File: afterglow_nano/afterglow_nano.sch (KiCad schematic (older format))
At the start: 64 parts, among them J1 J137_IN_C, J2 J133_IN_R, J3 Conn_Power, J4 J137_OUT_C, J5 J133_OUT_R, Q1 2N3904, Q10 FQP27P06, Q11 FQP27P06, Q12 FQP27P06, Q13 FQP27P06, Q14 FQP27P06, Q15 FQP27P06, Q16 FQP27P06, Q17 FQP30N06L, Q18 FQP30N06L, Q19 FQP30N06L, Q2 2N3904, Q20 FQP30N06L, Q21 FQP30N06L, Q22 FQP30N06L, Q23 FQP30N06L, Q24 FQP30N06L, Q3 2N3904, Q4 2N3904, Q5 2N3904, Q6 2N3904, Q7 2N3904, Q8 2N3904, Q9 FQP27P06, SW1 CFG, U1 74LS165, U2 74LS165, U3 5V_Regulator, U4 arduino_nano, U5 74HC595, U6 74HC595

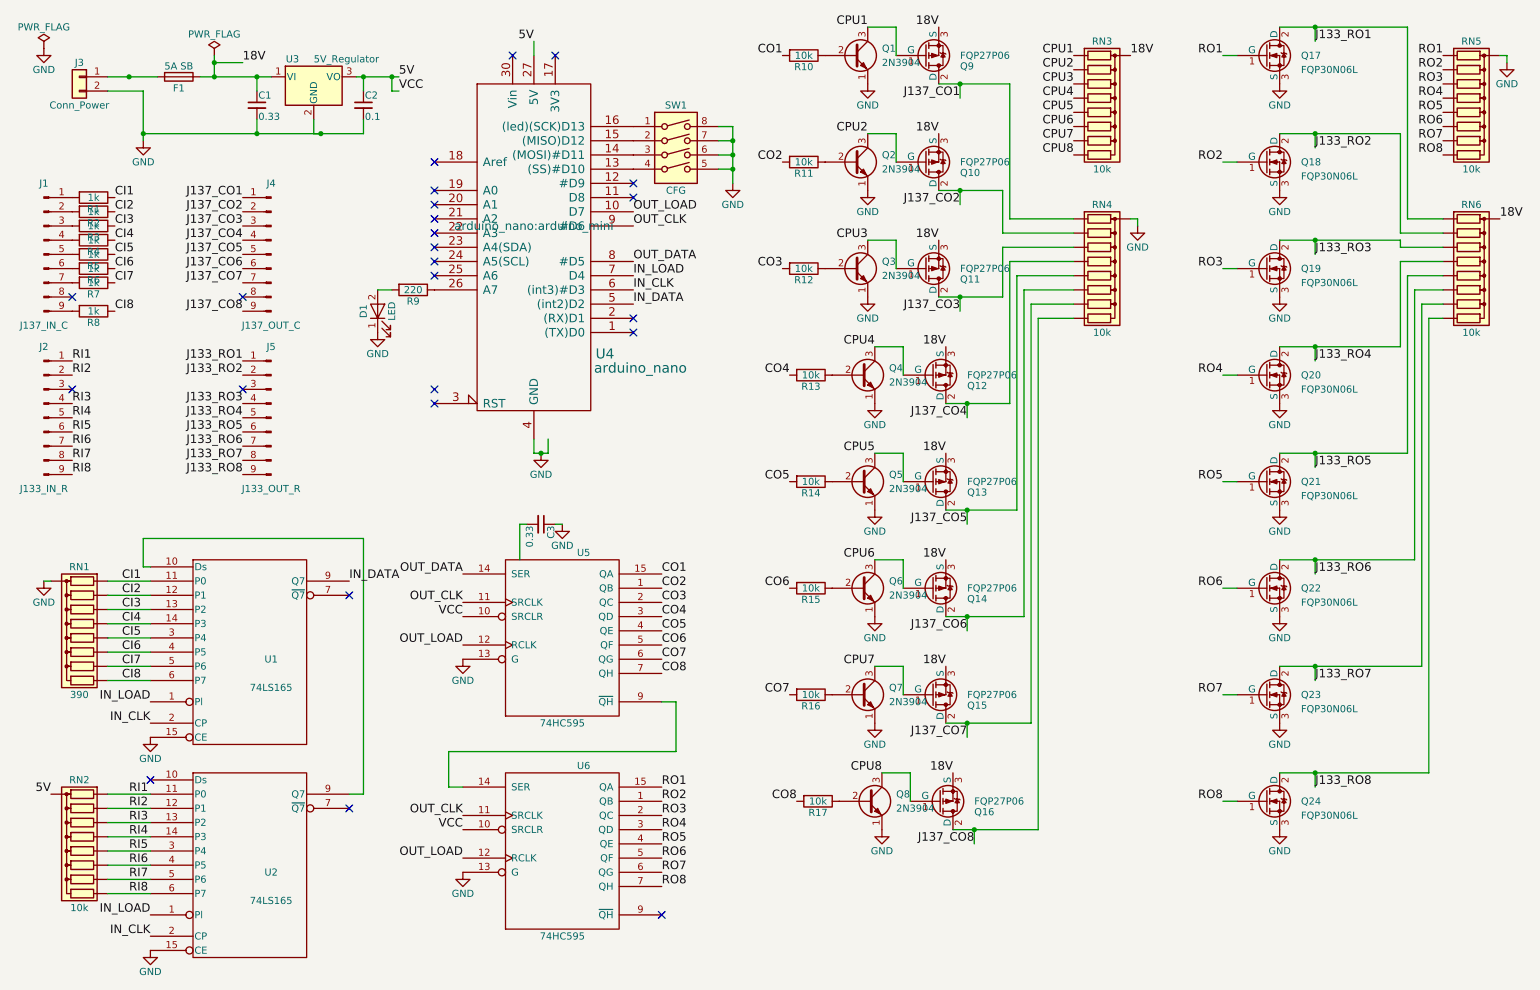
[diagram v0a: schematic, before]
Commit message: v1.1 schematic preparations
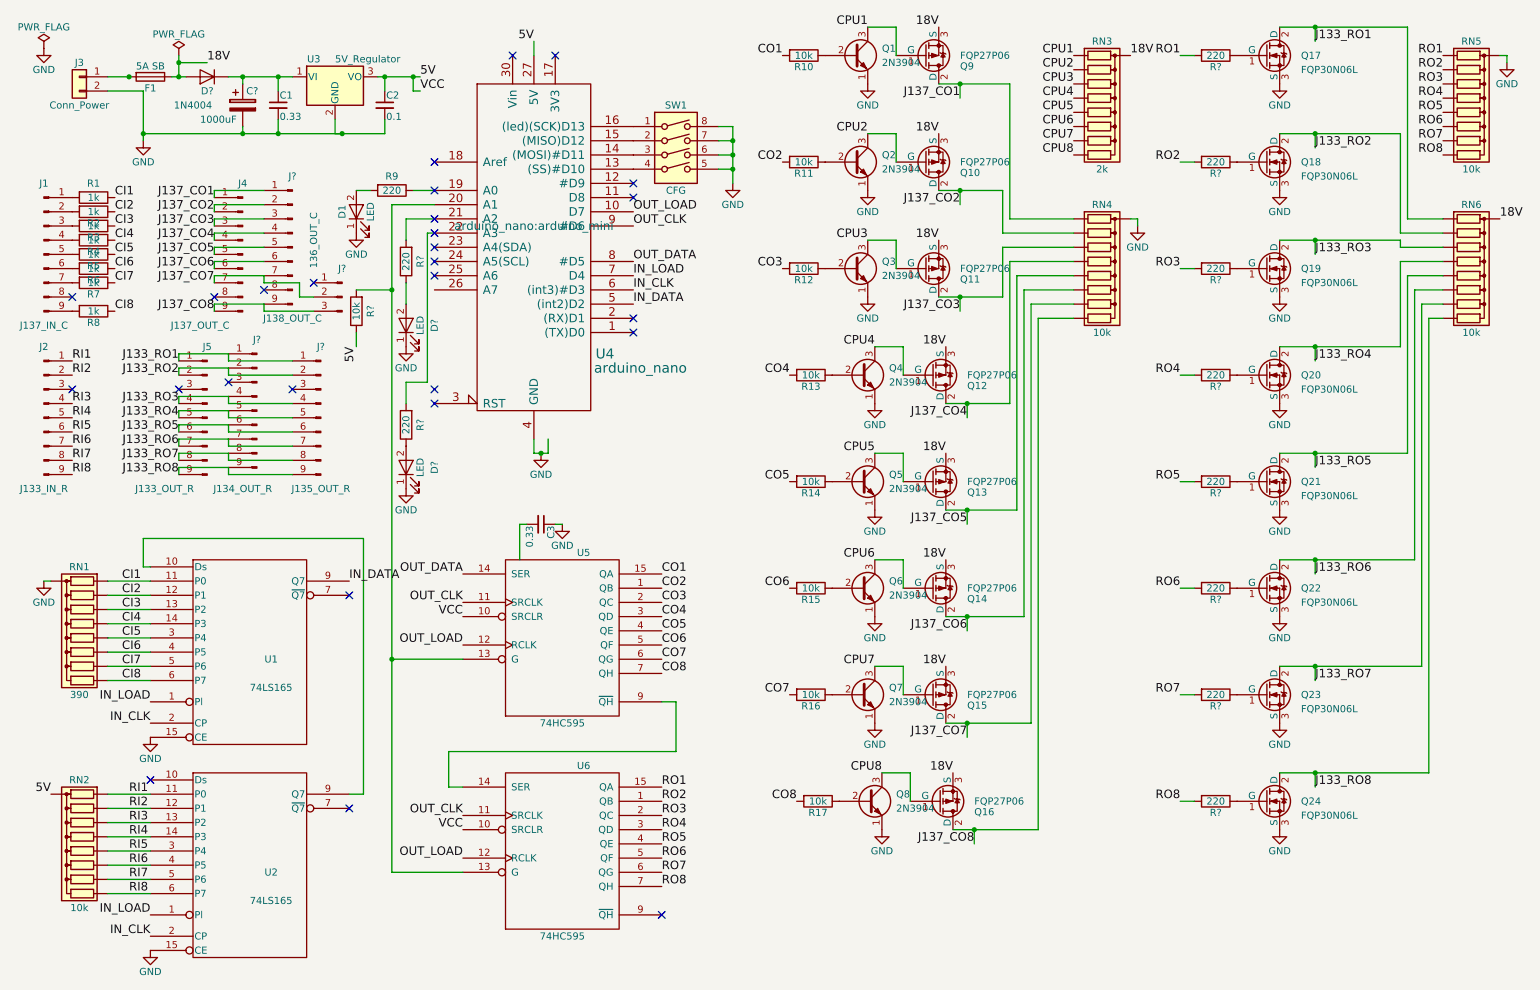
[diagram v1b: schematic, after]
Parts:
- added C?: 1000uF, symbol CP
- added D?: 1N4004, symbol D
- added D? (x2): LED, LEDs:LED_0805_HandSoldering, symbol LED
- added J?: J138_OUT_C, Connectors_Molex:Molex_KK-41791-9_9x3.96mm_Straight, symbol Conn_01x09_Male
- added J?: J134_OUT_R, Connectors_Molex:Molex_KK-6410-09_09x2.54mm_Straight, symbol Conn_01x09_Male
- added J?: J135_OUT_R, Connectors_Molex:Molex_KK-6410-09_09x2.54mm_Straight, symbol Conn_01x09_Male
- added J?: 136_OUT_C, symbol Conn_01x03_Male
- added R? (x8): 220, symbol R
- added R?: 10k, Resistors_SMD:R_0805_HandSoldering, symbol R
- added R? (x2): 220, Resistors_SMD:R_0805_HandSoldering, symbol R
- RN3: value 10k -> 2k
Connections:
- net 18V: now also D?.2 (A); no longer C1.1, U3.1 (VI)
- net GND: now also C?.2, D?.1 (K), D?.1 (K); no longer U5.13 (G), U6.13 (G)
- net J133_RO1: now also J?.1 (Pin_1), J?.1 (Pin_1)
- net J133_RO2: now also J?.2 (Pin_2), J?.2 (Pin_2)
- net J133_RO3: now also J?.4 (Pin_4), J?.4 (Pin_4)
- net J133_RO4: now also J?.5 (Pin_5), J?.5 (Pin_5)
- net J133_RO5: now also J?.6 (Pin_6), J?.6 (Pin_6)
- net J133_RO6: now also J?.7 (Pin_7), J?.7 (Pin_7)
- net J133_RO7: now also J?.8 (Pin_8), J?.8 (Pin_8)
- net J133_RO8: now also J?.9 (Pin_9), J?.9 (Pin_9)
- net J137_CO1: now also J?.1 (Pin_1)
- net J137_CO2: now also J?.2 (Pin_2)
- net J137_CO3: now also J?.3 (Pin_3)
- net J137_CO4: now also J?.4 (Pin_4)
- net J137_CO5: now also J?.5 (Pin_5)
- net J137_CO6: now also J?.6 (Pin_6)
- net J137_CO7: now also J?.2 (Pin_2), J?.7 (Pin_7)
- net J137_CO8: now also J?.3 (Pin_3), J?.9 (Pin_9)
- net RO1: now also R?.2; no longer Q17.1 (G)
- net RO2: now also R?.2; no longer Q18.1 (G)
- net RO3: now also R?.2; no longer Q19.1 (G)
- net RO4: now also R?.2; no longer Q20.1 (G)
- net RO5: now also R?.2; no longer Q21.1 (G)
- net RO6: now also R?.2; no longer Q22.1 (G)
- net RO7: now also R?.2; no longer Q23.1 (G)
- net RO8: now also R?.2; no longer Q24.1 (G)
- net VCC: now also R?.1
- net at U4.19 (A0): now also R9.1
- net at U4.20 (A1): now also U5.13 (G), U6.13 (G), R?.2
- net at U4.21 (A2): now also R?.2
- net at U4.22 (A3): now also R?.2
- net at U4.26 (A7): no longer R9.1
- new net: C1.1, C?.1, D?.1 (K), U3.1 (VI)
- new net: Q17.1 (G), R?.1
- new net: Q18.1 (G), R?.1
- new net: Q19.1 (G), R?.1
- new net: Q20.1 (G), R?.1
- new net: Q21.1 (G), R?.1
- new net: Q22.1 (G), R?.1
- new net: Q23.1 (G), R?.1
- new net: Q24.1 (G), R?.1
- new net: D?.2 (A), R?.1 (x2)
- no-connect marks 24 -> 27
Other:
- moved on the sheet: C1, C2, D1, F1, J4, J5, R9, U3
